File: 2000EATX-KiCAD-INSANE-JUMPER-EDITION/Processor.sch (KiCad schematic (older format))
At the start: 19 parts, among them U100 MC68000, U103 74HCT245, U104 74HCT373, U105 74HCT245, U106 74HCT373, U303 74HCT08

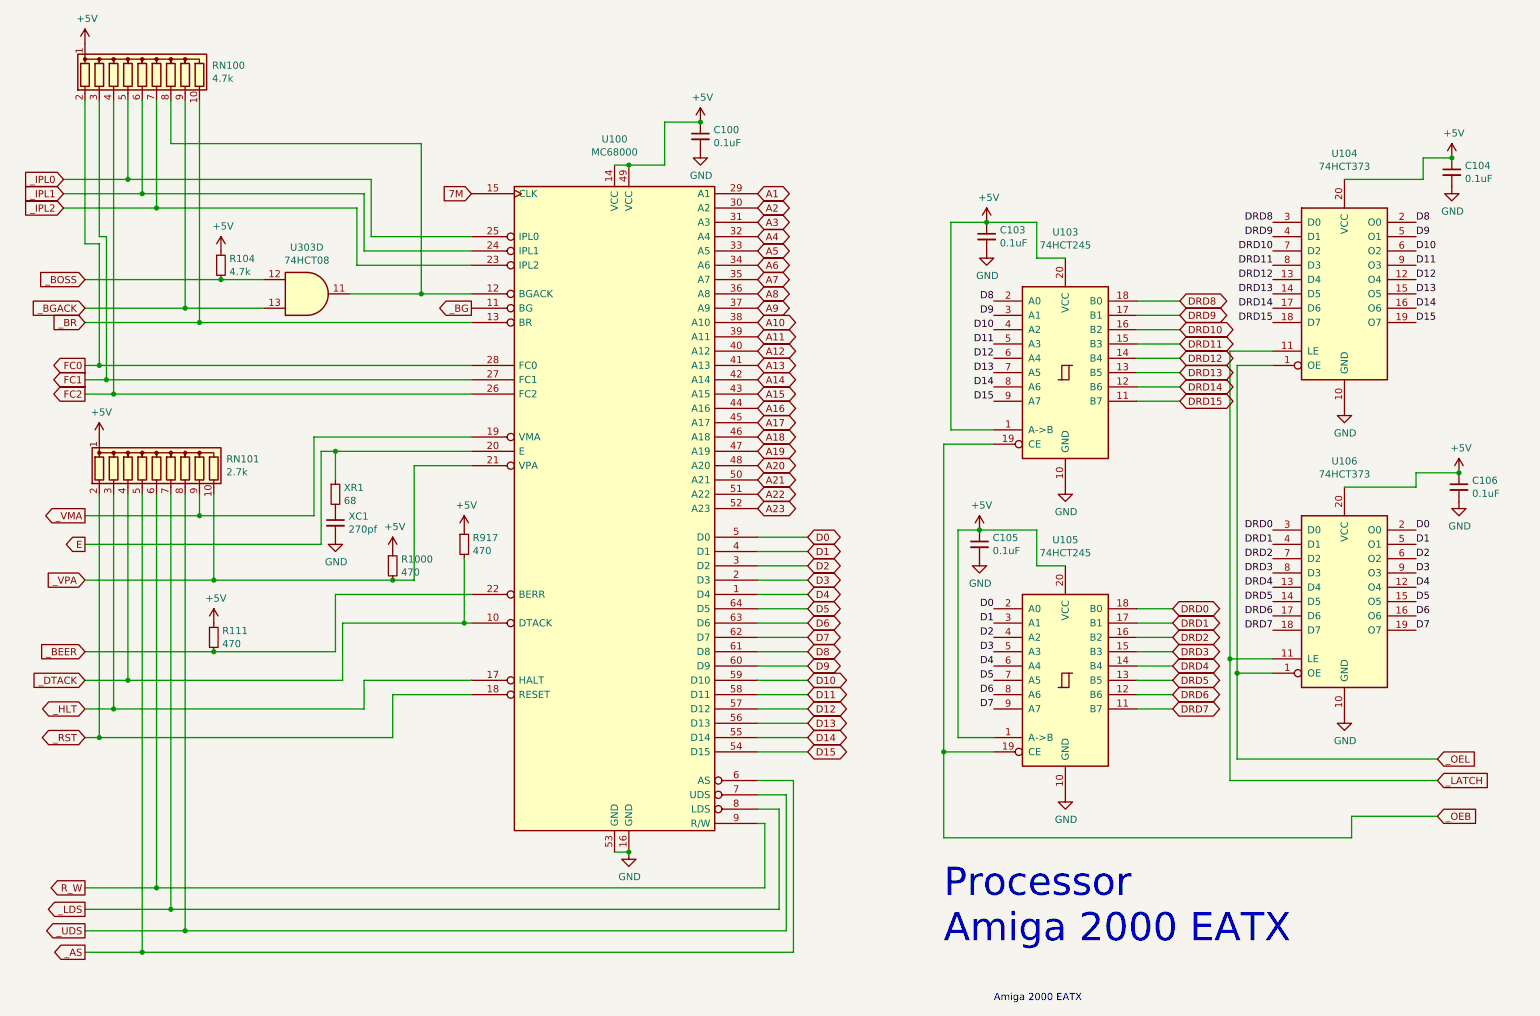
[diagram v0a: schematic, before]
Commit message: Add files via upload
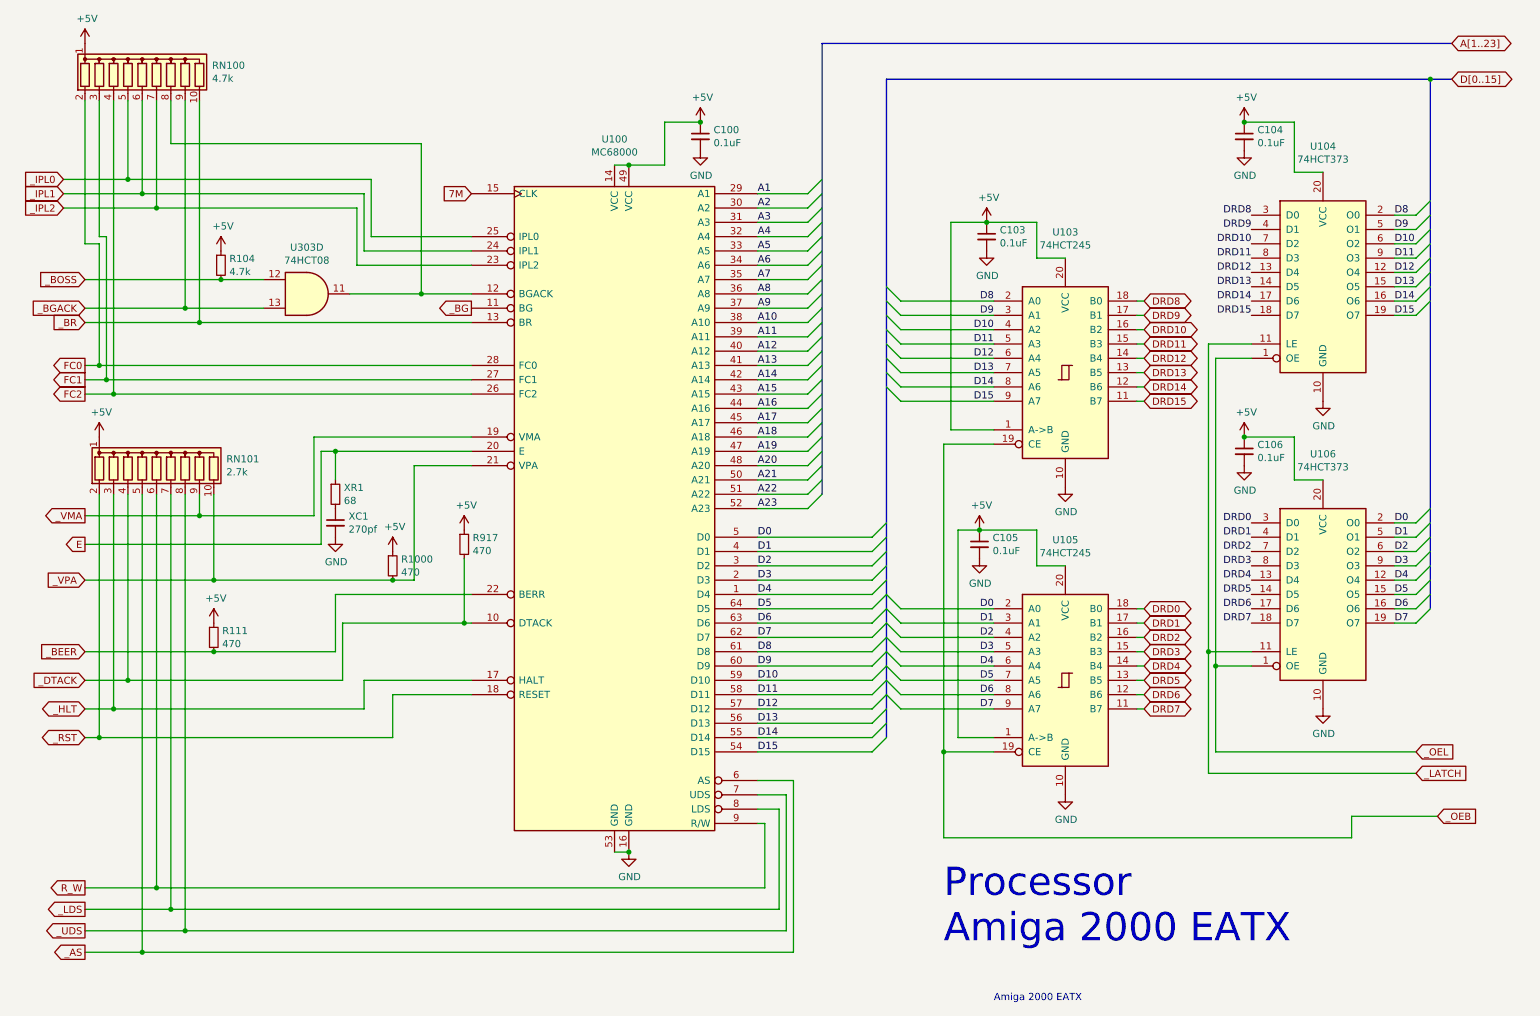
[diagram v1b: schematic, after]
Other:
- moved on the sheet: C104, C106, U104, U106

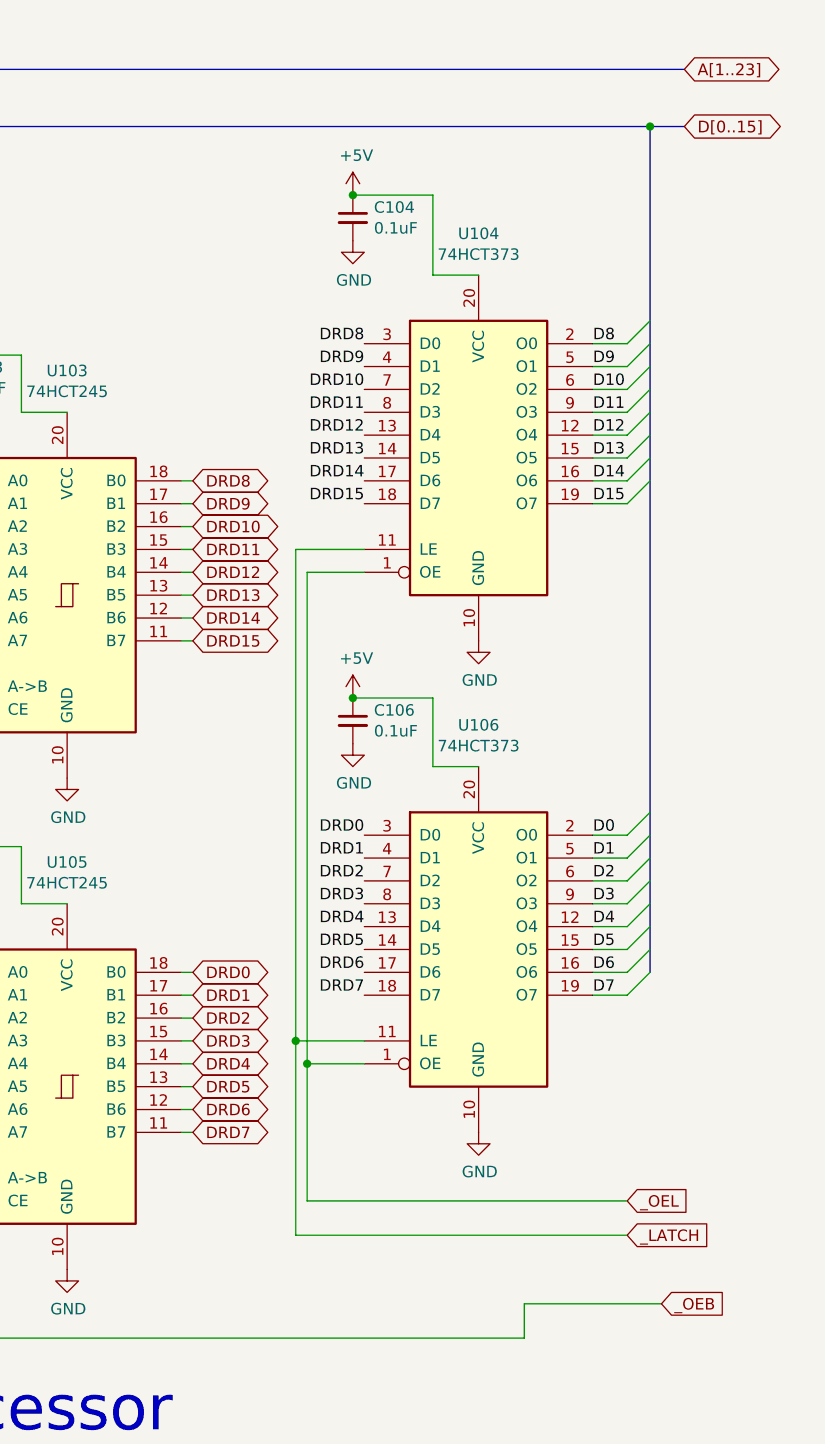
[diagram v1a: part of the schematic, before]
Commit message: Add files via upload
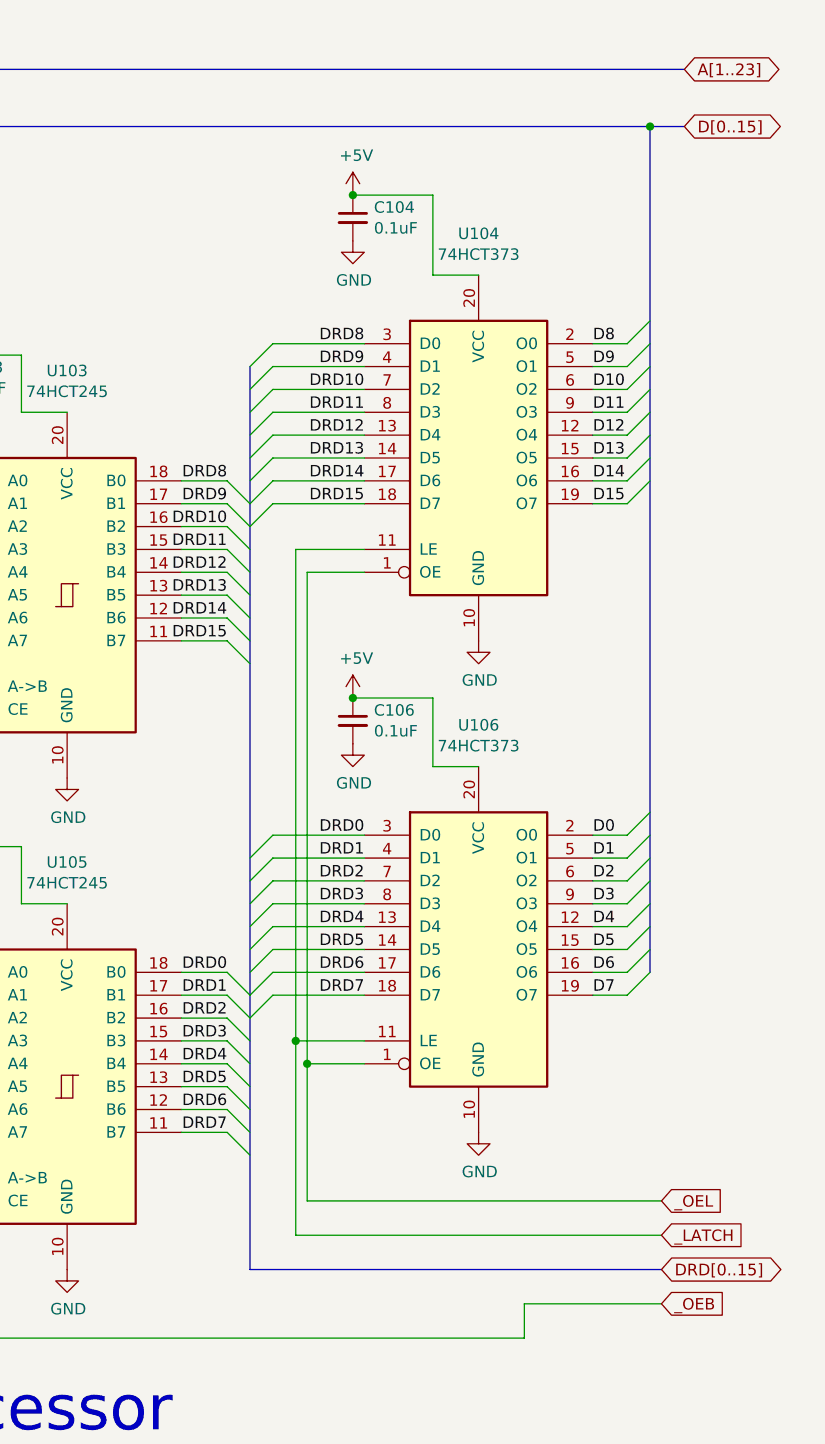
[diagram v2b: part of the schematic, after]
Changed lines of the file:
@@
 	5750 5750 6550 5750
 Wire Wire Line
-	8400 5450 8450 5450
-Wire Wire Line
-	8400 5350 8450 5350
-Wire Wire Line
-	8400 5250 8450 5250
-Wire Wire Line
-	8400 5150 8450 5150
-Wire Wire Line
-	8400 5050 8450 5050
-Wire Wire Line
-	8400 4950 8450 4950
-Wire Wire Line
-	8400 4850 8450 4850
-Wire Wire Line
-	8400 4750 8450 4750
-Text GLabel 8450 5450 2    50   BiDi ~ 0
-DRD7
-Text GLabel 8450 5350 2    50   BiDi ~ 0
-DRD6
-Text GLabel 8450 5250 2    50   BiDi ~ 0
-DRD5
-Text GLabel 8450 5150 2    50   BiDi ~ 0
-DRD4
-Text GLabel 8450 5050 2    50   BiDi ~ 0
-DRD3
-Text GLabel 8450 4950 2    50   BiDi ~ 0
-DRD2
-Text GLabel 8450 4850 2    50   BiDi ~ 0
-DRD1
-Text GLabel 8450 4750 2    50   BiDi ~ 0
-DRD0
-Wire Wire Line
-	8400 2600 8450 2600
-Wire Wire Line
-	8400 2700 8450 2700
-Wire Wire Line
-	8400 2800 8450 2800
-Wire Wire Line
-	8400 2900 8450 2900
-Wire Wire Line
-	8400 3000 8450 3000
-Wire Wire Line
-	8400 3100 8450 3100
-Wire Wire Line
-	8400 3200 8450 3200
-Wire Wire Line
-	8400 3300 8450 3300
-Text GLabel 8450 2600 2    50   BiDi ~ 0
-DRD8
-Text GLabel 8450 2700 2    50   BiDi ~ 0
-DRD9
-Text GLabel 8450 2800 2    50   BiDi ~ 0
-DRD10
-Text GLabel 8450 2900 2    50   BiDi ~ 0
-DRD11
-Text GLabel 8450 3000 2    50   BiDi ~ 0
-DRD12
-Text GLabel 8450 3100 2    50   BiDi ~ 0
-DRD13
-Text GLabel 8450 3200 2    50   BiDi ~ 0
-DRD14
-Text GLabel 8450 3300 2    50   BiDi ~ 0
-DRD15
+	8400 5450 8600 5450
+Wire Wire Line
+	8400 5350 8600 5350
+Wire Wire Line
+	8400 5250 8600 5250
+Wire Wire Line
+	8400 5150 8600 5150
+Wire Wire Line
+	8400 5050 8600 5050
+Wire Wire Line
+	8400 4950 8600 4950
+Wire Wire Line
+	8400 4850 8600 4850
+Wire Wire Line
+	8400 4750 8600 4750
+Wire Wire Line
+	8400 2600 8600 2600
+Wire Wire Line
+	8400 2700 8600 2700
+Wire Wire Line
+	8400 2800 8600 2800
+Wire Wire Line
+	8400 2900 8600 2900
+Wire Wire Line
+	8400 3000 8600 3000
+Wire Wire Line
+	8400 3100 8600 3100
+Wire Wire Line
+	8400 3200 8600 3200
+Wire Wire Line
+	8400 3300 8600 3300
 Text GLabel 900  1750 0    50   Input ~ 0
 _IPL0
@@
 Text Notes 7400 7500 0    50   ~ 0
 Amiga 2000 EATX
-Text GLabel 10350 5900 2    50   Input ~ 0
+Text GLabel 10500 5900 2    50   Input ~ 0
 _LATCH
 Wire Wire Line
 	9200 2900 8900 2900
 Wire Wire Line
-	8900 2900 8900 5050
-Wire Wire Line
-	8900 5900 10350 5900
+	8900 5900 10500 5900
 Wire Wire Line
 	9200 5050 8900 5050
@@
 Wire Wire Line
 	8900 5050 8900 5900
-Text GLabel 10350 5750 2    50   Input ~ 0
+Text GLabel 10500 5750 2    50   Input ~ 0
 _OEL
 Wire Wire Line
@@
 	8950 3000 8950 5150
 Wire Wire Line
-	8950 5750 10350 5750
+	8950 5750 10500 5750
 Wire Wire Line
 	9200 5150 8950 5150
@@
 Entry Wire Line
 	10350 4850 10450 4750
-Wire Bus Line
-	10450 4750 10450 1050
 Connection ~ 10450 1050
 Wire Bus Line
@@
 Wire Wire Line
 	10200 2700 10350 2700
+Entry Wire Line
+	10350 2000 10450 1900
+Entry Wire Line
+	10350 2100 10450 2000
+Entry Wire Line
+	10350 2200 10450 2100
+Entry Wire Line
+	10350 2300 10450 2200
+Entry Wire Line
+	10350 2400 10450 2300
+Entry Wire Line
+	10350 2500 10450 2400
+Entry Wire Line
+	10350 2600 10450 2500
+Entry Wire Line
+	10350 2700 10450 2600
+Entry Wire Line
+	10350 4150 10450 4050
+Entry Wire Line
+	10350 4250 10450 4150
+Entry Wire Line
+	10350 4350 10450 4250
+Entry Wire Line
+	10350 4450 10450 4350
+Entry Wire Line
+	10350 4750 10450 4650
+Entry Wire Line
+	10350 4650 10450 4550
+Entry Wire Line
+	10350 4550 10450 4450
+Wire Wire Line
+	9200 2000 8800 2000
+Entry Wire Line
+	8800 2000 8700 2100
+Wire Bus Line
+	8700 6050 10500 6050
+Text GLabel 10500 6050 2    51   BiDi ~ 0
+DRD[0..15]
+Entry Wire Line
+	8600 2600 8700 2700
+Text Label 8600 2600 2    50   ~ 0
+DRD8
+Text Label 8600 2700 2    50   ~ 0
+DRD9
+Text Label 8600 2800 2    50   ~ 0
+DRD10
+Text Label 8600 2900 2    50   ~ 0
+DRD11
+Text Label 8600 3000 2    50   ~ 0
+DRD12
+Text Label 8600 3100 2    50   ~ 0
+DRD13
+Text Label 8600 3200 2    50   ~ 0
+DRD14
+Text Label 8600 3300 2    50   ~ 0
+DRD15
+Entry Wire Line
+	8600 2700 8700 2800
+Entry Wire Line
+	8600 2800 8700 2900
+Entry Wire Line
+	8600 2900 8700 3000
+Entry Wire Line
+	8600 3000 8700 3100
+Entry Wire Line
+	8600 3100 8700 3200
+Entry Wire Line
+	8600 3200 8700 3300
+Entry Wire Line
+	8600 3300 8700 3400
+Wire Wire Line
+	9200 2700 8800 2700
+Wire Wire Line
+	9200 2600 8800 2600
+Wire Wire Line
+	9200 2500 8800 2500
+Wire Wire Line
+	9200 2400 8800 2400
+Wire Wire Line
+	9200 2300 8800 2300
+Wire Wire Line
+	9200 2200 8800 2200
+Wire Wire Line
+	9200 2100 8800 2100
+Entry Wire Line
+	8800 2700 8700 2800
+Entry Wire Line
+	8800 2600 8700 2700
+Entry Wire Line
+	8800 2500 8700 2600
+Entry Wire Line
+	8800 2400 8700 2500
+Entry Wire Line
+	8800 2300 8700 2400
+Entry Wire Line
+	8800 2200 8700 2300
+Entry Wire Line
+	8800 2100 8700 2200
+Wire Wire Line
+	9200 4150 8800 4150
+Entry Wire Line
+	8800 4850 8700 4950
+Entry Wire Line
+	8800 4750 8700 4850
+Entry Wire Line
+	8800 4650 8700 4750
+Entry Wire Line
+	8800 4550 8700 4650
+Entry Wire Line
+	8800 4450 8700 4550
+Entry Wire Line
+	8800 4350 8700 4450
+Entry Wire Line
+	8800 4250 8700 4350
+Entry Wire Line
+	8800 4150 8700 4250
+Wire Wire Line
+	8800 4250 9200 4250
+Wire Wire Line
+	8800 4350 9200 4350
+Wire Wire Line
+	8800 4450 9200 4450
+Wire Wire Line
+	8800 4550 9200 4550
+Wire Wire Line
+	8800 4650 9200 4650
+Wire Wire Line
+	8800 4750 9200 4750
+Wire Wire Line
+	8800 4850 9200 4850
+Wire Wire Line
+	8900 2900 8900 5050
+Wire Bus Line
+	10450 1050 10450 4750
 Wire Bus Line
 	6200 800  6200 3950
 Wire Bus Line
 	6650 1050 6650 5650
-Entry Wire Line
-	10350 2000 10450 1900
-Entry Wire Line
-	10350 2100 10450 2000
-Entry Wire Line
-	10350 2200 10450 2100
-Entry Wire Line
-	10350 2300 10450 2200
-Entry Wire Line
-	10350 2400 10450 2300
-Entry Wire Line
-	10350 2500 10450 2400
-Entry Wire Line
-	10350 2600 10450 2500
-Entry Wire Line
-	10350 2700 10450 2600
-Entry Wire Line
-	10350 4150 10450 4050
-Entry Wire Line
-	10350 4250 10450 4150
-Entry Wire Line
-	10350 4350 10450 4250
-Entry Wire Line
-	10350 4450 10450 4350
-Entry Wire Line
-	10350 4750 10450 4650
-Entry Wire Line
-	10350 4650 10450 4550
-Entry Wire Line
-	10350 4550 10450 4450
+Wire Bus Line
+	8700 2100 8700 6050
+Entry Wire Line
+	8600 4750 8700 4850
+Entry Wire Line
+	8600 5450 8700 5550
+Entry Wire Line
+	8600 5350 8700 5450
+Entry Wire Line
+	8600 5250 8700 5350
+Entry Wire Line
+	8600 5150 8700 5250
+Entry Wire Line
+	8600 5050 8700 5150
+Entry Wire Line
+	8600 4950 8700 5050
+Entry Wire Line
+	8600 4850 8700 4950
+Text Label 8600 4750 2    50   ~ 0
+DRD0
+Text Label 8600 4850 2    50   ~ 0
+DRD1
+Text Label 8600 4950 2    50   ~ 0
+DRD2
+Text Label 8600 5050 2    50   ~ 0
+DRD3
+Text Label 8600 5150 2    50   ~ 0
+DRD4
+Text Label 8600 5250 2    50   ~ 0
+DRD5
+Text Label 8600 5350 2    50   ~ 0
+DRD6
+Text Label 8600 5450 2    50   ~ 0
+DRD7
 $EndSCHEMATC
